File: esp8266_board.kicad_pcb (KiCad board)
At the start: 2 copper layers, 76.2 x 50.8 mm, 11 parts, among them P1 CONN_01X11, P2 CONN_01X11, U1 ESP-12F, U2 AP111733

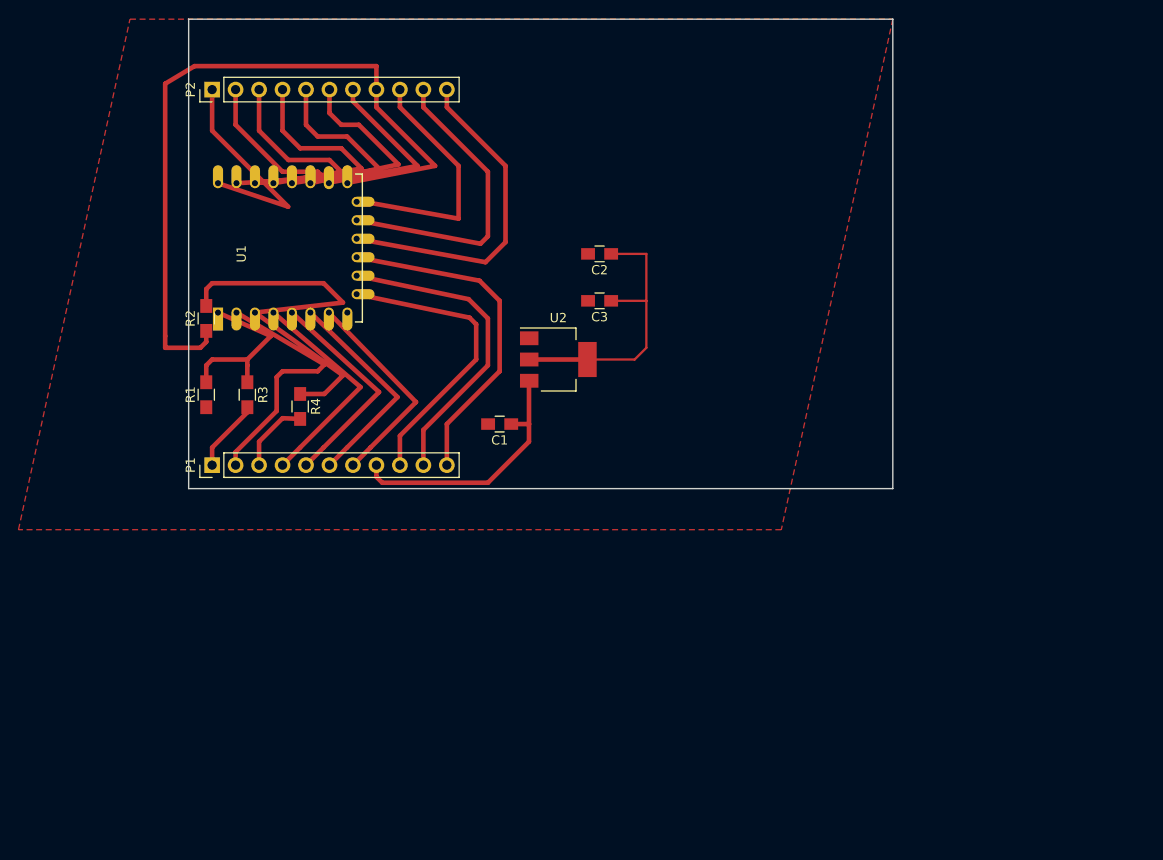
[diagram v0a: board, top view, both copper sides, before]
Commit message: v1
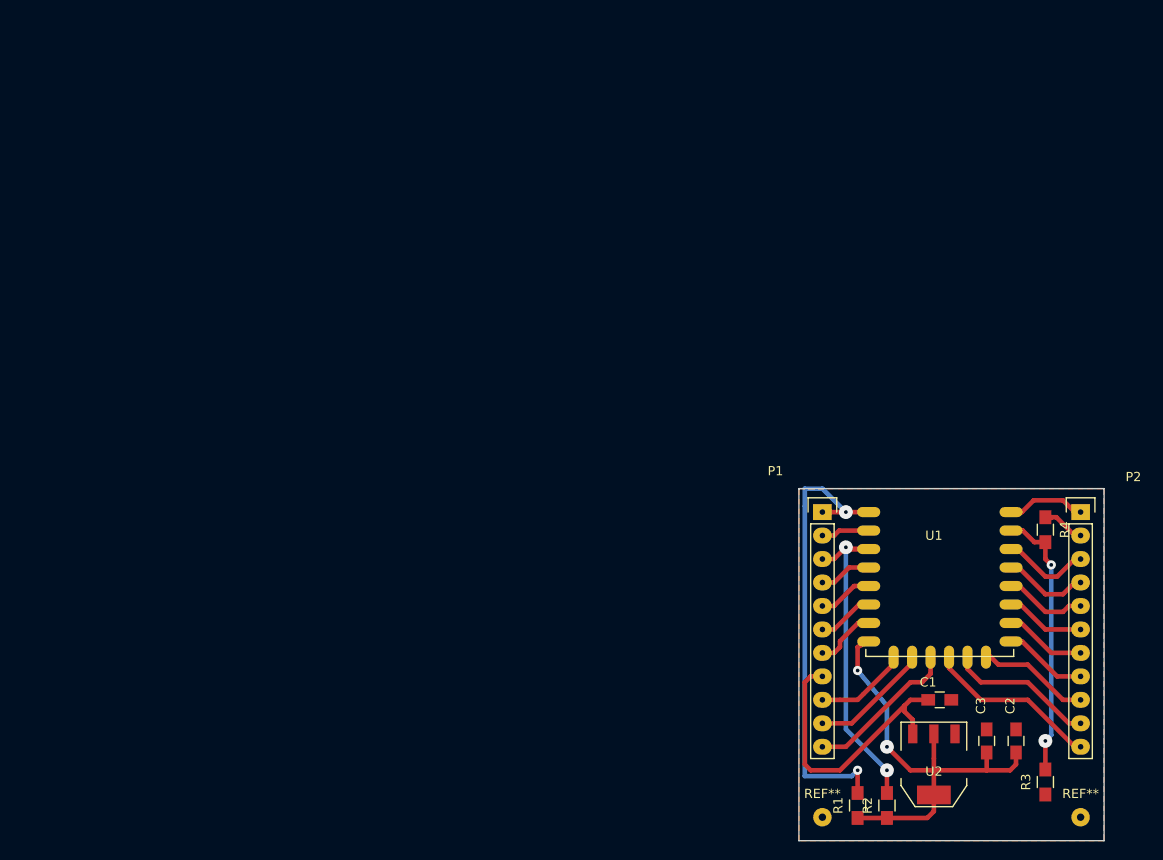
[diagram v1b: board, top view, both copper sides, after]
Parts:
- added REF**: drill, Wire_Pads:SolderWirePad_single_0-8mmDrill, F.Cu at (119.4, 111.8)
- added REF**: drill, Wire_Pads:SolderWirePad_single_0-8mmDrill, F.Cu at (147.3, 111.8)
- P1, P2: footprint Pin_Headers:Pin_Header_Straight_1x11_Pitch2.54mm -> Pin_Headers:Pin_Header_Straight_1x11
- R1, R2: value 2k -> 10k
- R3: value 1k -> 2k
- U1: footprint ESP8266:ESP-12E -> ESP8266:ESP-12F
- U2: value AP111733 -> AMS1117-3V3
- moved P2 104.5 mm to (147.3, 78.7), turned to 0 degrees
- moved R3 96.0 mm to (143.5, 108.0), turned to 90 degrees
- moved R2 90.6 mm to (126.4, 110.5)
- moved R1 83.3 mm to (123.2, 110.5)
- moved R4 81.7 mm to (143.5, 80.6)
- moved U1 74.3 mm to (125.1, 78.7), turned to 0 degrees
- moved C2 69.3 mm to (140.3, 103.5), turned to 90 degrees
- moved P1 66.2 mm to (119.4, 78.7), turned to 0 degrees
- moved C3 63.4 mm to (137.2, 103.5), turned to 90 degrees
- moved U2 59.8 mm to (131.4, 106.0), turned to 180 degrees
- moved C1 56.2 mm to (132.1, 99.1), turned to 0 degrees
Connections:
- C2 pad 1: Net-(C2-Pad1) -> +3V3
- C3 pad 1: Net-(C2-Pad1) -> +3V3
- R1 pad 1: GND -> +3V3
- R1 pad 2: Net-(R1-Pad2) -> Net-(P1-Pad1)
- R2 pad 1: GND -> +3V3
- R2 pad 2: Net-(R2-Pad2) -> Net-(P1-Pad3)
- R3 pad 1: Net-(R1-Pad2) -> GND
- R3 pad 2: Net-(P1-Pad1) -> Net-(R3-Pad2)
- R4 pad 1: Net-(R2-Pad2) -> Net-(P2-Pad2)
- R4 pad 2: Net-(P1-Pad3) -> Net-(R3-Pad2)
- U1 pad 1: Net-(R1-Pad2) -> Net-(P1-Pad1)
- U1 pad 15: Net-(P2-Pad2) -> Net-(R3-Pad2)
- U1 pad 3: Net-(R2-Pad2) -> Net-(P1-Pad3)
- U1 pad 8: Net-(C2-Pad1) -> +3V3
- U2 pad 2: Net-(C2-Pad1) -> +3V3
- U2 pad 4: Net-(C2-Pad1) -> +3V3
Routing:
- net GND: track 87.5 -> 9.79 mm
- net +3V3: track 0.00 -> 49.4 mm, vias 0 -> 2
- net Net-(R2-Pad2): track 44.5 -> 0.00 mm
- net Net-(P1-Pad1): track 7.85 -> 51.4 mm, vias 0 -> 2
- net Net-(C2-Pad1): track 31.0 -> 0.00 mm
- net Net-(P1-Pad3): track 8.04 -> 38.2 mm, vias 0 -> 2
- net Net-(R3-Pad2): track 0.00 -> 30.1 mm, vias 0 -> 2
- net Net-(P1-Pad2): track 28.2 -> 5.94 mm
- net Net-(P1-Pad9): track 32.2 -> 10.7 mm
- net Net-(P1-Pad10): track 34.1 -> 13.7 mm
- net Net-(P1-Pad11): track 36.8 -> 17.5 mm
- net Net-(R1-Pad2): track 18.8 -> 0.00 mm
- net Net-(P1-Pad4): track 24.4 -> 6.39 mm
- net Net-(P2-Pad10): track 33.6 -> 16.6 mm
- net Net-(P2-Pad7): track 25.8 -> 9.57 mm
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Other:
- board size 76.2 x 50.8 mm -> 33 x 38.1 mm
- net class Default: via_dia 0.6 -> 1.5
- rule trace_min: 0.2 -> 0.4
- rule via_min_drill: 0.3 -> 0.4
- rule via_min_size: 0.4 -> 1.5
